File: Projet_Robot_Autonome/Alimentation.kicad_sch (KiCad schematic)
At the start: 28 parts, among them IC1 MP1475DJ-LF-P, J2 Screw_Terminal_01x02, SW1 ON/OFF

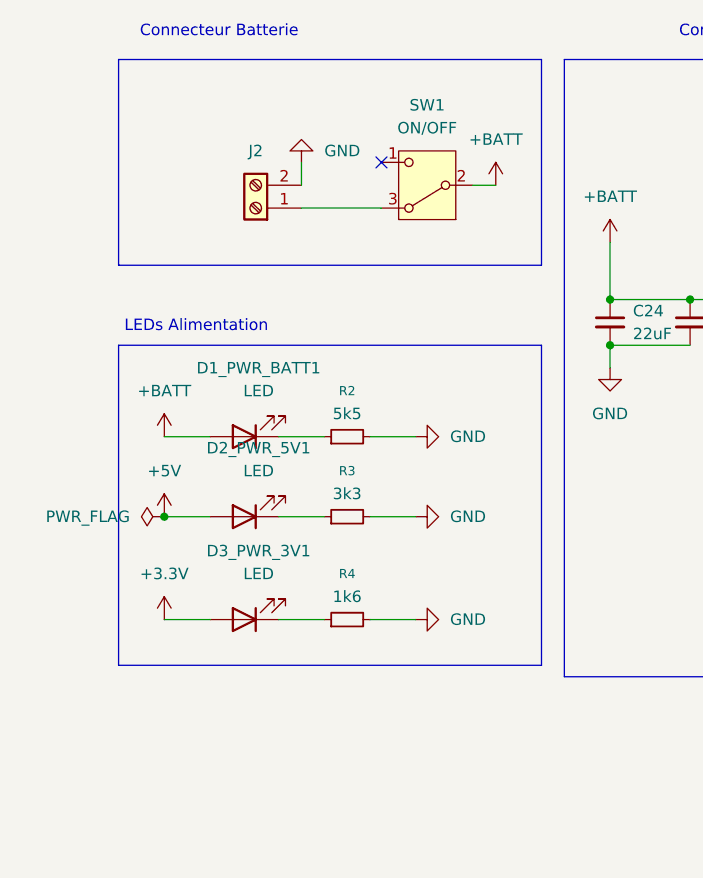
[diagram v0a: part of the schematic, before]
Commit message: Updated KiCad project files
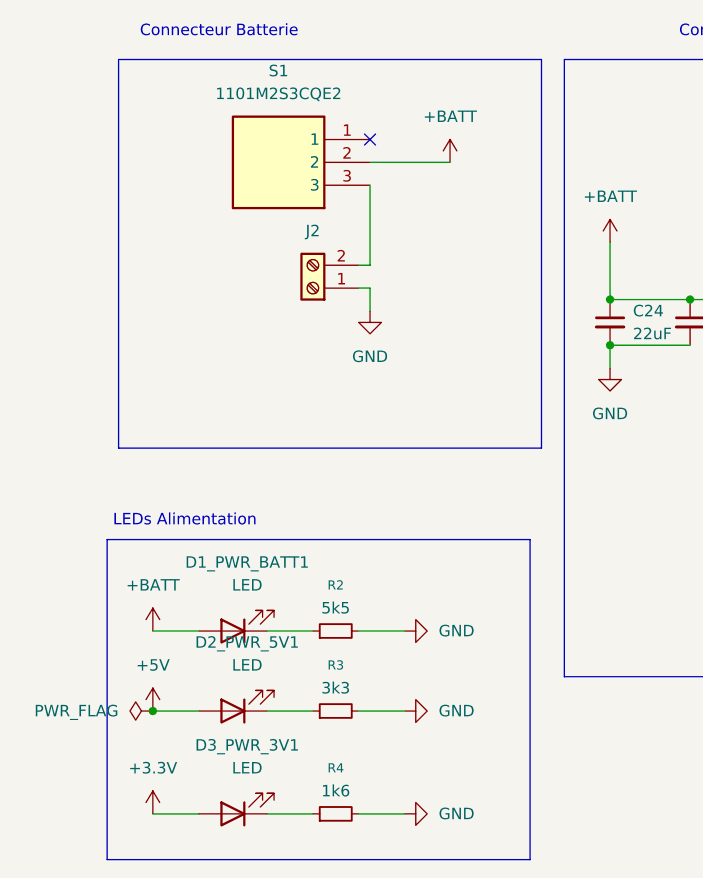
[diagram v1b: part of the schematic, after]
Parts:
- removed SW1: ON/OFF, Button_Switch_SMD:Nidec_Copal_CAS-120A, symbol Switch:SW_Nidec_CAS-120A1
- added S1: 1101M2S3CQE2, swithes:sw wurth, symbol 1101M2S3CQE2:1101M2S3CQE2
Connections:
- net +BATT: now also S1.2
- net GND: now also J2.1 (Pin_1); no longer J2.2 (Pin_2)
- new net: J2.2 (Pin_2), S1.3
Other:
- moved on the sheet: D1_PWR_BATT1, D2_PWR_5V1, D3_PWR_3V1, J2, R2, R3, R4
